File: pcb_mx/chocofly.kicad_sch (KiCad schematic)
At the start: 133 parts, among them P1 battery+, P2 battery-, SW1 SW_Push, SW11 SW_Push, SW12 SW_Push, SW13 SW_Push, SW14 SW_Push, SW15 SW_Push, SW16 SW_Push, SW17 SW_Push, SW18 SW_Push, SW19 SW_Push, SW2 SW_Push, SW20 SW_Push, SW21 SW_Push, SW22 SW_Push, SW23 SW_Push, SW24 SW_Push, SW25 SW_Push, SW26 SW_Push, SW27 SW_Push, SW28 SW_Push, SW29 SW_Push, SW3 SW_Push, SW30 SW_Push, SW31 SW_Push, SW32 SW_Push, SW33 SW_Push, SW34 SW_Push, SW35 SW_Push, SW36 SW_Push, SW37 SW_Push, SW38 SW_Push, SW39 SW_Push, SW4 SW_Push, SW40 SW_Push, SW41 SW_Push, SW42 SW_Push, SW43 SW_Push, SW44 SW_Push, SW45 SW_Push, SW46 SW_Push, SW47 SW_Push, SW48 SW_Push, SW49 SW_Push, SW5 SW_Push, SW50 SW_Push, SW51 SW_Push, SW52 SW_Push, SW53 SW_Push, SW54 SW_Push, SW55 SW_Push, SW56 SW_Push, SW57 SW_Push, SW58 SW_Push, SW59 SW_Push, SW6 SW_Push, SW60 SW_Push, SW61 SW_Push, SW62 Reset, SW63 Power, SW7 SW_Push, SW8 SW_Push, SW9 SW_Push

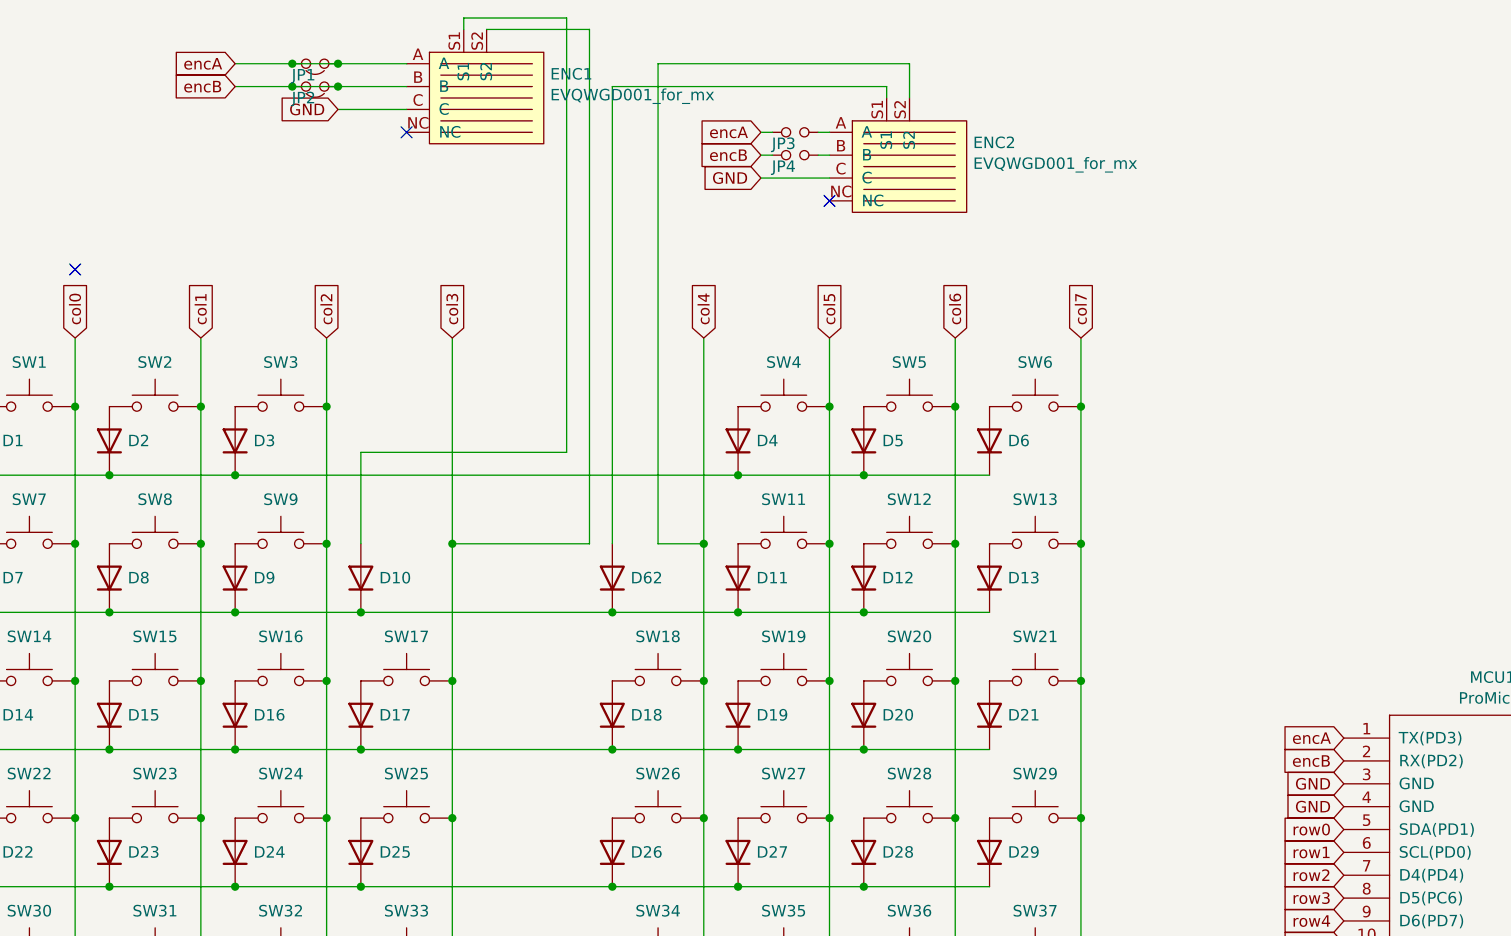
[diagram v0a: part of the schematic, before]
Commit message: wip on chocomx
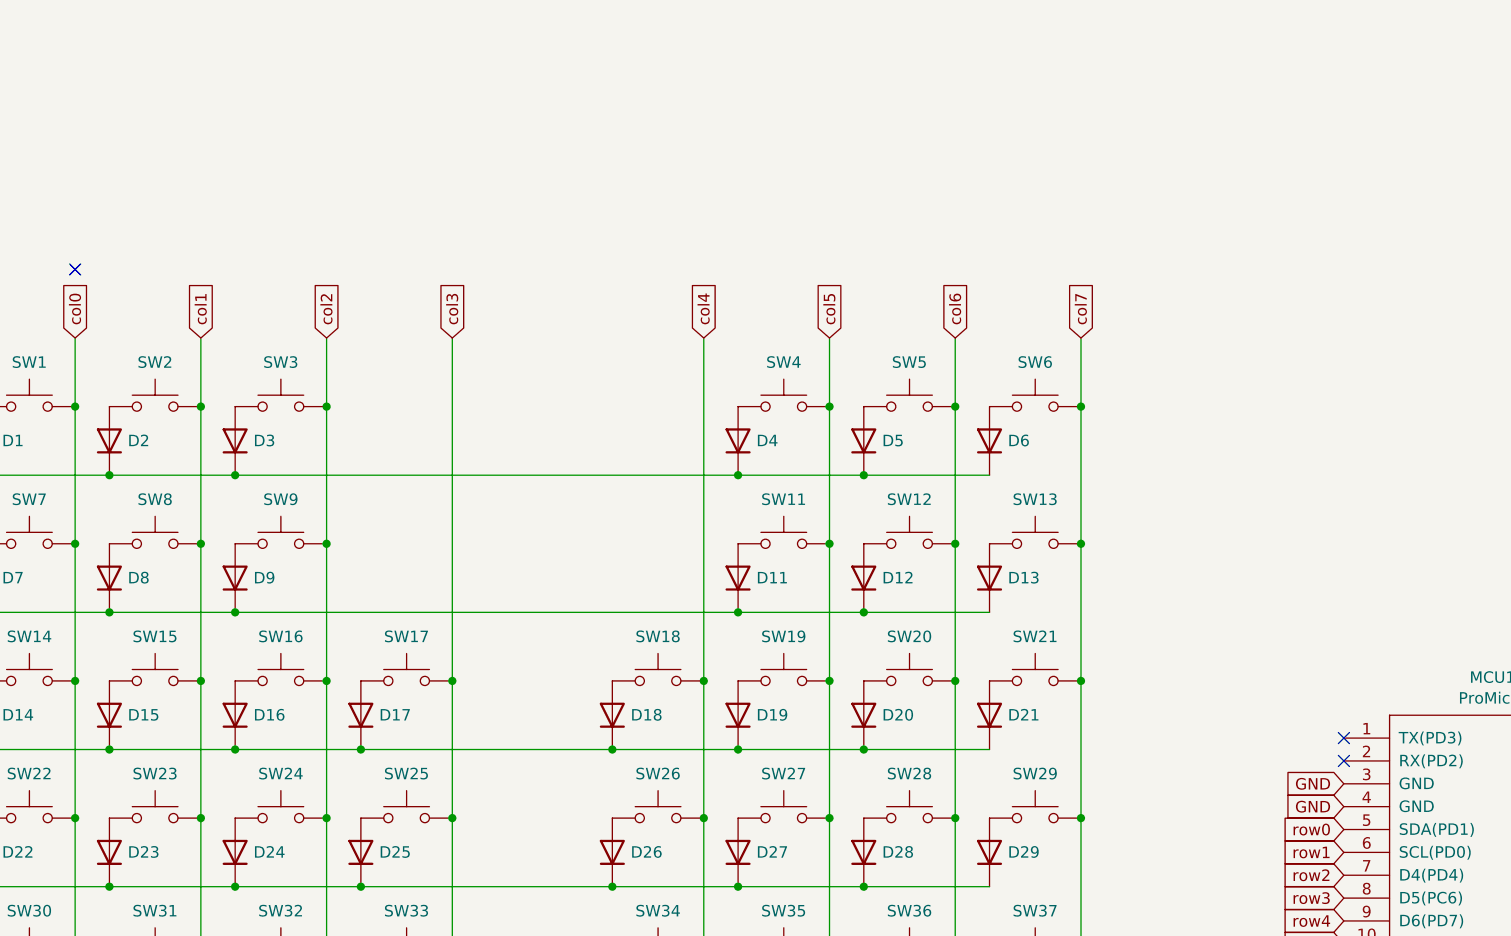
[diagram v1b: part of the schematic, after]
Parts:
- removed D10, D62: 1N4148, footprints:diode_TH_SMD, symbol Diode:1N4148
- removed ENC1, ENC2: EVQWGD001_for_mx, footprints:EVQWGD001_for_mx, symbol chocofly-rescue:EVQWGD001-evqwgd001
- removed JP1, JP2: Jumper_NC_Small, footprints:avalanche_Jumper_NC, symbol chocofly-rescue:Jumper_NC_Small-Device
- removed JP3, JP4: Jumper_NC_Small, footprints:avalanche_Jumper, symbol chocofly-rescue:Jumper_NO_Small-Device
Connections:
- net encA: no longer names the net of MCU1.1 (TX(PD3))
- net encB: no longer names the net of MCU1.2 (RX(PD2))
